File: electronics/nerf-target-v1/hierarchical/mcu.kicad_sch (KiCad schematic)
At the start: 21 parts, among them J3 CortexDebug10, SW1 reset, U1 W25Q128JVS, U2 RP2040, Y1 X322512MSB4SI

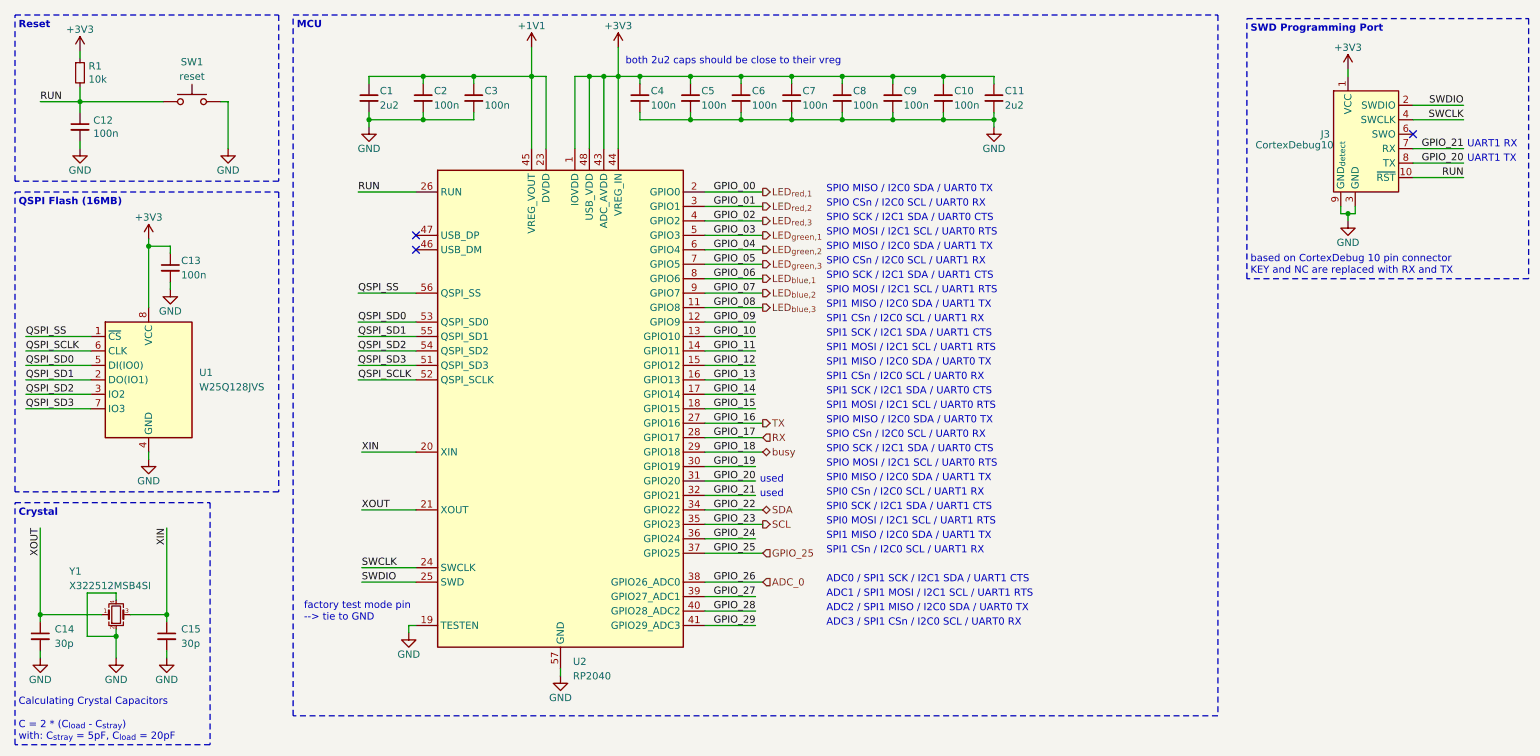
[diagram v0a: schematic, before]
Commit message: finished board; production files
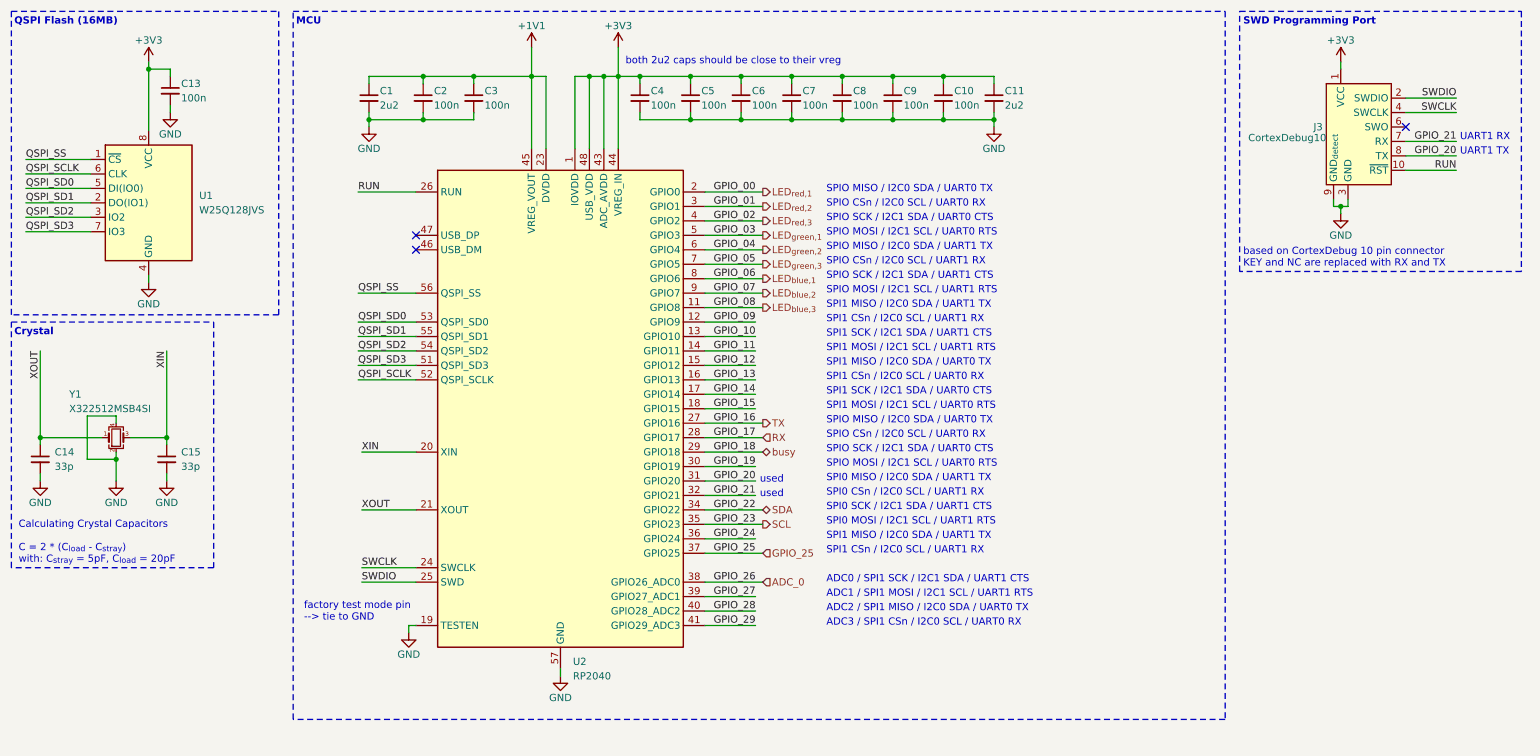
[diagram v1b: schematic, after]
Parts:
- removed C12: 100n, Capacitor_SMD:C_0402_1005Metric, symbol Device:C_Small
- removed R1: 10k, Resistor_SMD:R_0603_1608Metric, symbol Device:R_Small
- removed SW1: reset, Button_Switch_SMD:SW_SPST_TL3342, symbol Switch:SW_Push
- C14, C15: value 30p -> 33p; LCSC Part # C1570 -> C1562
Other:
- note removed: "Reset"
- moved on the sheet: C13, C14, C15, J3, U1, Y1
